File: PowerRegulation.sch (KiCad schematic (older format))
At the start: 6 parts, among them U301 LM2931D-R

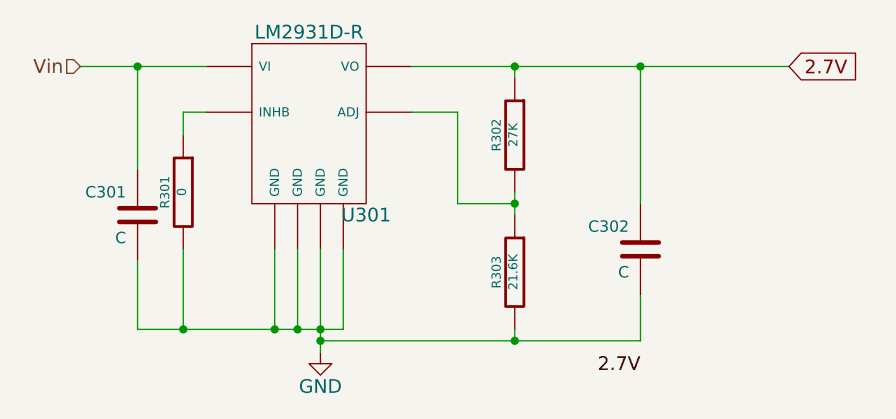
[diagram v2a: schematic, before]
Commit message: test netlist
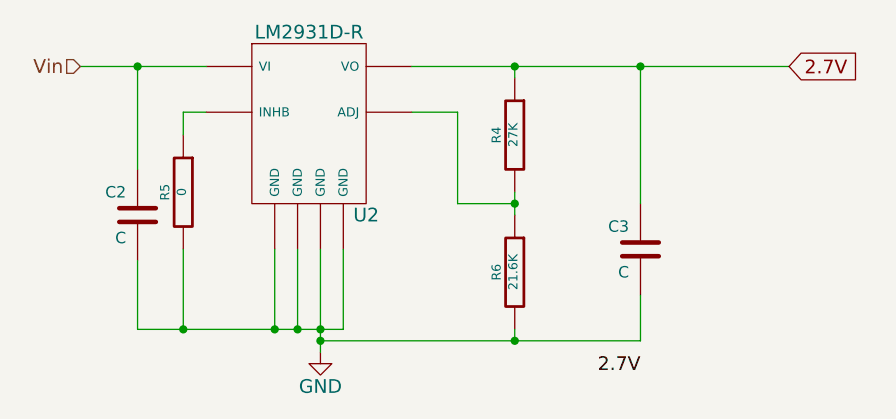
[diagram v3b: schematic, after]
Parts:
- renumbered C301 to C2, C302 to C3, R302 to R4, R301 to R5, R303 to R6, U301 to U2
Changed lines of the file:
@@
 $EndDescr
 $Comp
-L GND #PWR06
+L GND #PWR6
 U 1 1 54DAF107
 P 4800 3900
-F 0 "#PWR06" H 4800 3650 60  0001 C CNN
+F 0 "#PWR6" H 4800 3650 60  0001 C CNN
 F 1 "GND" H 4800 3750 60  0000 C CNN
 F 2 "" H 4800 3900 60  0000 C CNN
@@
 $EndComp
 $Comp
-L C C301
+L C C2
 U 1 1 54DAF10D
 P 4000 3300
-F 0 "C301" H 4050 3400 50  0000 L CNN
+F 0 "C2" H 4050 3400 50  0000 L CNN
 F 1 "C" H 4050 3200 50  0000 L CNN
 F 2 "SMD_Packages:SMD-0805" H 4038 3150 30  0001 C CNN
@@
 $EndComp
 $Comp
-L C C302
+L C C3
 U 1 1 54DAF114
 P 6200 3450
-F 0 "C302" H 6250 3550 50  0000 L CNN
+F 0 "C3" H 6250 3550 50  0000 L CNN
 F 1 "C" H 6250 3350 50  0000 L CNN
 F 2 "SMD_Packages:SMD-0805" H 6238 3300 30  0001 C CNN
@@
 	4000 3800 4000 3500
 $Comp
-L R R301
+L R R5
 U 1 1 54DAF11D
 P 4200 3200
-F 0 "R301" V 4280 3200 40  0000 C CNN
+F 0 "R5" V 4280 3200 40  0000 C CNN
 F 1 "0" V 4207 3201 40  0000 C CNN
 F 2 "SMD_Packages:SMD-0805" V 4130 3200 30  0001 C CNN
@@
 2.7V
 $Comp
-L LM2931D-R U301
+L LM2931D-R U2
 U 1 1 54DAF12F
 P 4750 3150
-F 0 "U301" H 5000 3000 60  0000 C CNN
+F 0 "U2" H 5000 3000 60  0000 C CNN
 F 1 "LM2931D-R" H 4750 3800 60  0000 C CNN
 F 2 "SMD_Packages:SOIC-8-N" H 4600 3150 60  0001 C CNN
@@
 Connection ~ 6200 2650
 $Comp
-L R R302
+L R R4
 U 1 1 54DAF13B
 P 5650 2950
-F 0 "R302" V 5730 2950 40  0000 C CNN
+F 0 "R4" V 5730 2950 40  0000 C CNN
 F 1 "27K" V 5657 2951 40  0000 C CNN
 F 2 "SMD_Packages:SMD-0805" V 5580 2950 30  0001 C CNN
@@
 $EndComp
 $Comp
-L R R303
+L R R6
 U 1 1 54DAF142
 P 5650 3550
-F 0 "R303" V 5730 3550 40  0000 C CNN
+F 0 "R6" V 5730 3550 40  0000 C CNN
 F 1 "21.6K" V 5657 3551 40  0000 C CNN
 F 2 "SMD_Packages:SMD-0805" V 5580 3550 30  0001 C CNN

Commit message: Routing done - Final
Just add artwork
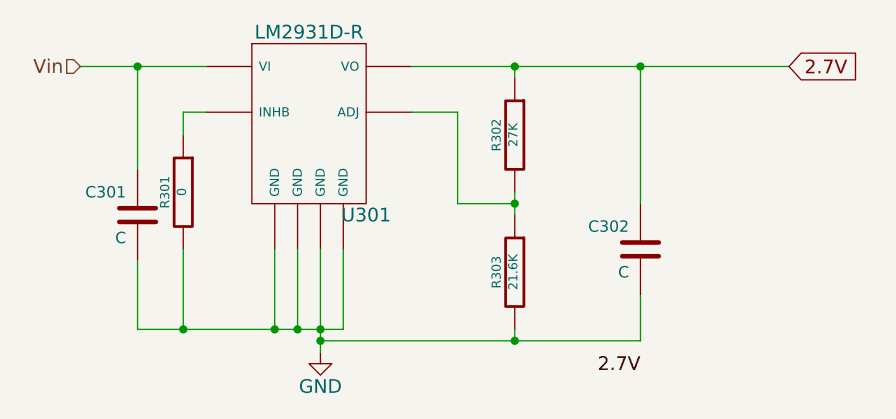
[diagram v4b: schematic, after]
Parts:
- renumbered C2 to C301, C3 to C302, R5 to R301, R4 to R302, R6 to R303, U2 to U301
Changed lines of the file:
@@
 $EndDescr
 $Comp
-L GND #PWR6
+L GND #PWR06
 U 1 1 54DAF107
 P 4800 3900
-F 0 "#PWR6" H 4800 3650 60  0001 C CNN
+F 0 "#PWR06" H 4800 3650 60  0001 C CNN
 F 1 "GND" H 4800 3750 60  0000 C CNN
 F 2 "" H 4800 3900 60  0000 C CNN
@@
 $EndComp
 $Comp
-L C C2
+L C C301
 U 1 1 54DAF10D
 P 4000 3300
-F 0 "C2" H 4050 3400 50  0000 L CNN
+F 0 "C301" H 4050 3400 50  0000 L CNN
 F 1 "C" H 4050 3200 50  0000 L CNN
 F 2 "SMD_Packages:SMD-0805" H 4038 3150 30  0001 C CNN
@@
 $EndComp
 $Comp
-L C C3
+L C C302
 U 1 1 54DAF114
 P 6200 3450
-F 0 "C3" H 6250 3550 50  0000 L CNN
+F 0 "C302" H 6250 3550 50  0000 L CNN
 F 1 "C" H 6250 3350 50  0000 L CNN
 F 2 "SMD_Packages:SMD-0805" H 6238 3300 30  0001 C CNN
@@
 	4000 3800 4000 3500
 $Comp
-L R R5
+L R R301
 U 1 1 54DAF11D
 P 4200 3200
-F 0 "R5" V 4280 3200 40  0000 C CNN
+F 0 "R301" V 4280 3200 40  0000 C CNN
 F 1 "0" V 4207 3201 40  0000 C CNN
 F 2 "SMD_Packages:SMD-0805" V 4130 3200 30  0001 C CNN
@@
 2.7V
 $Comp
-L LM2931D-R U2
+L LM2931D-R U301
 U 1 1 54DAF12F
 P 4750 3150
-F 0 "U2" H 5000 3000 60  0000 C CNN
+F 0 "U301" H 5000 3000 60  0000 C CNN
 F 1 "LM2931D-R" H 4750 3800 60  0000 C CNN
 F 2 "SMD_Packages:SOIC-8-N" H 4600 3150 60  0001 C CNN
@@
 Connection ~ 6200 2650
 $Comp
-L R R4
+L R R302
 U 1 1 54DAF13B
 P 5650 2950
-F 0 "R4" V 5730 2950 40  0000 C CNN
+F 0 "R302" V 5730 2950 40  0000 C CNN
 F 1 "27K" V 5657 2951 40  0000 C CNN
 F 2 "SMD_Packages:SMD-0805" V 5580 2950 30  0001 C CNN
@@
 $EndComp
 $Comp
-L R R6
+L R R303
 U 1 1 54DAF142
 P 5650 3550
-F 0 "R6" V 5730 3550 40  0000 C CNN
+F 0 "R303" V 5730 3550 40  0000 C CNN
 F 1 "21.6K" V 5657 3551 40  0000 C CNN
 F 2 "SMD_Packages:SMD-0805" V 5580 3550 30  0001 C CNN
